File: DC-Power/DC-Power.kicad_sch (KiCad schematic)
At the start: 0 parts

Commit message: Draw Type-c
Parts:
- added U1: TYPE-C_16PLC-H10_0, JLCImport:TYPE-C_16PLC-H10_0, symbol JLCImport:TYPE-C_16PLC-H10_0
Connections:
- new net +VDC: U1.A4 (VBUS), U1.A9 (VBUS), U1.B4 (VBUS), U1.B9 (VBUS)
- new net CC1: U1.A5 (CC1)
- new net CC2: U1.B5 (CC2)
- new net D+: U1.A6 (D+), U1.B6 (D+)
- new net D-: U1.A7 (D-), U1.B7 (D-)
- new net GND: U1.1 (EH), U1.2 (EH), U1.3 (EH), U1.4 (EH), U1.A1 (GND), U1.A12 (GND), U1.B1 (GND), U1.B12 (GND)
- no-connect marks 0 -> 2

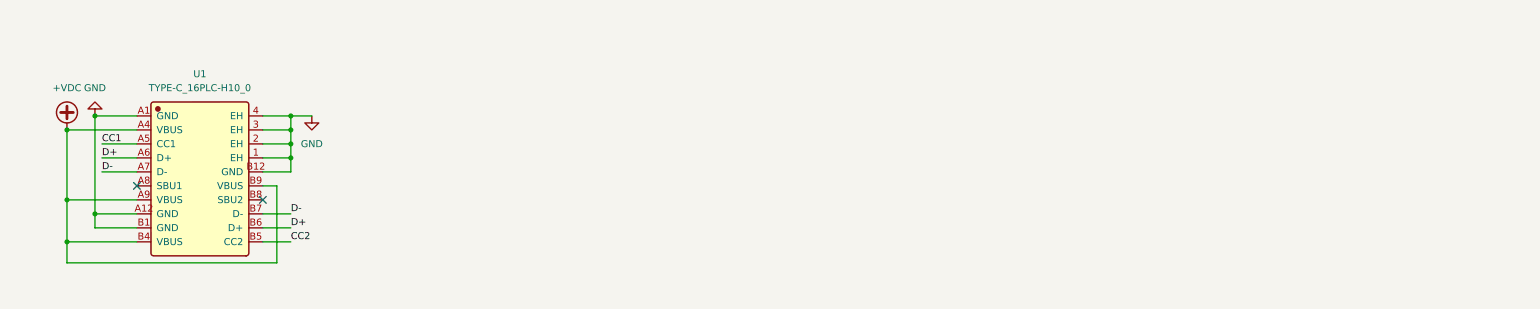
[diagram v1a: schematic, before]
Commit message: 5V,3.3V
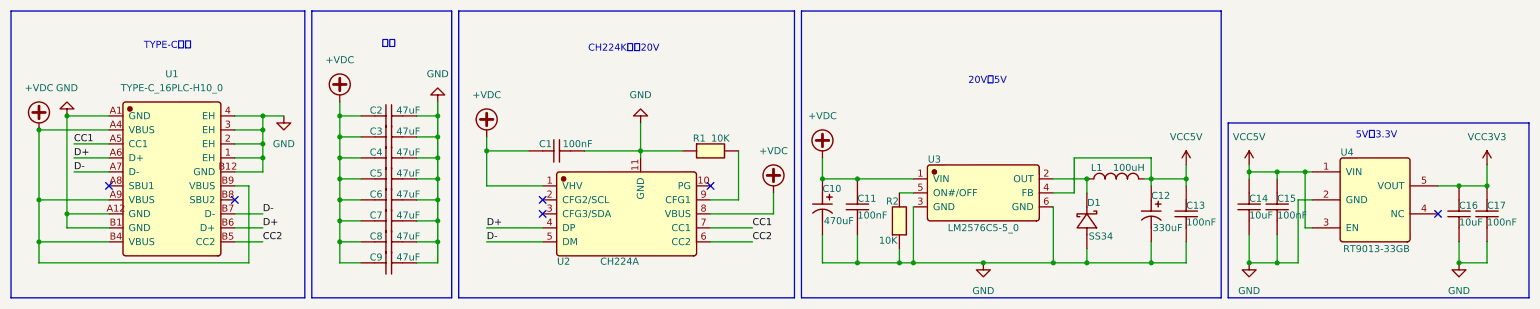
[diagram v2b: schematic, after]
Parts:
- added C1, C11, C13, C15, C17: 100nF, JLCImport:C0603, symbol JLCImport:C
- added C10: 470uF, JLCImport:MA35V470M10X13, symbol JLCImport:MA35V470M10X13
- added C12: 330uF, JLCImport:MA35V470M10X13, symbol JLCImport:MA35V470M10X13
- added C14, C16: 10uF, JLCImport:C0603, symbol JLCImport:C
- added C2, C3, C4, C5, C6, C7, C8, C9: 47uF, JLCImport:C1206, symbol JLCImport:C
- added D1: SS34, JLCImport:SS34_C7420365, symbol JLCImport:SS34_C7420365
- added L1: 100uH, JLCImport:PSPMAA1050H-101M-ANP, symbol JLCImport:PSPMAA1050H-101M-ANP
- added R1, R2: 10K, JLCImport:R0603, symbol JLCImport:R
- added U2: CH224A, JLCImport:CH224A, symbol JLCImport:CH224A
- added U3: LM2576C5-5_0, JLCImport:LM2576C5-5_0, symbol JLCImport:LM2576C5-5_0
- added U4: RT9013-33GB, JLCImport:RT9013-33GB, symbol JLCImport:RT9013-33GB
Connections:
- net +VDC: now also C1.1, C10.1, C11.2, C2.1, C3.1, C4.1, C5.1, C6.1, C7.1, C8.1, C9.1, U2.1 (VHV), U2.8 (VBUS), U3.1 (VIN)
- net CC1: now also U2.7 (CC1)
- net CC2: now also U2.6 (CC2)
- net D+: now also U2.4 (DP)
- net D-: now also U2.5 (DM)
- net GND: now also C1.2, C10.2, C11.1, C12.2, C13.1, C14.1, C15.1, C16.1, C17.1, C2.2, C3.2, C4.2, C5.2, C6.2, C7.2, C8.2, C9.2, D1.1 (A), R1.1, R2.1, U2.11 (GND), U3.3 (GND), U3.6 (GND), U4.2 (GND)
- new net: D1.2 (K), L1.1, U3.2 (OUT)
- new net: R2.2, U3.5 (ON#/OFF)
- new net: R1.2, U2.9 (CFG1)
- new net VCC3V3: C16.2, C17.2, U4.5 (VOUT)
- new net VCC5V: C12.1, C13.2, C14.2, C15.2, L1.2, U3.4 (FB), U4.1 (VIN), U4.3 (EN)
- no-connect marks 2 -> 6
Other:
- note added: "20V转5V"
- note added: "5V转3.3V"
- note added: "CH224K诱导20V"
- note added: "TYPE-C接口"
- note added: "滤波"
- moved on the sheet: U1
